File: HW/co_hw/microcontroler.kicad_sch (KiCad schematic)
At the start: 26 parts, among them J2 DS18B20, J3 DS18B20, J4 PRESSURE_SENSOR, J5 PWM, J7 Programmer, SW1 RotaryEncoder_Switch, SW2 SW_DIP_x03, SW3 SW_Push, U1 STM32F103C8Tx, U6 W25Q32JVSS, Y1 8Mhz

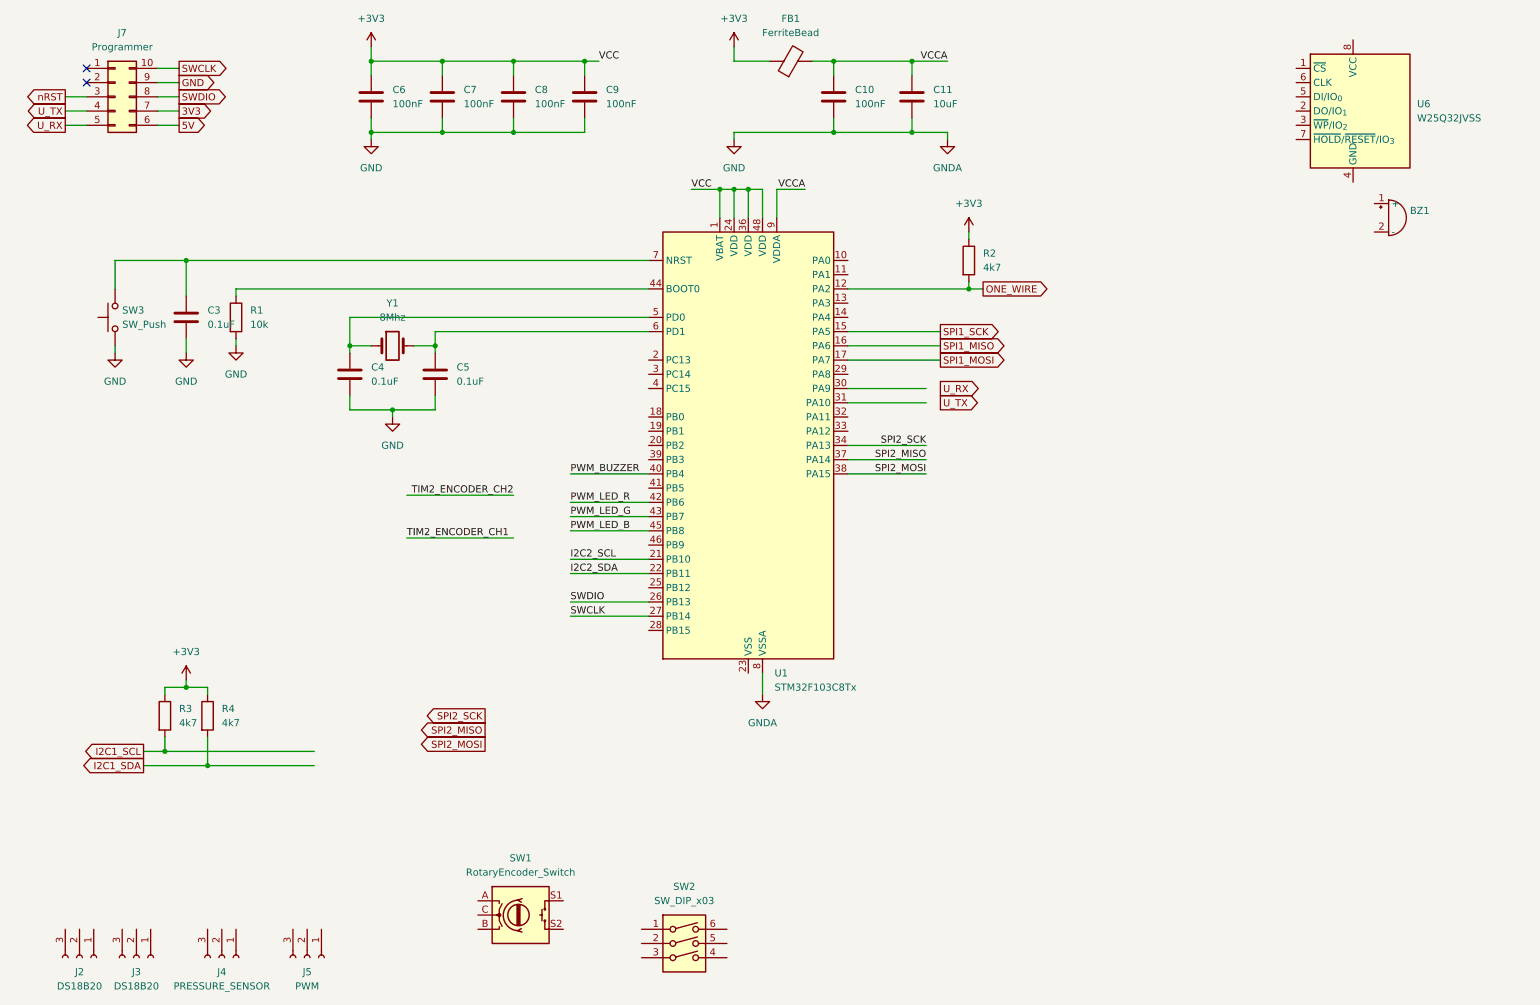
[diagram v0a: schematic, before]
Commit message: HW update.
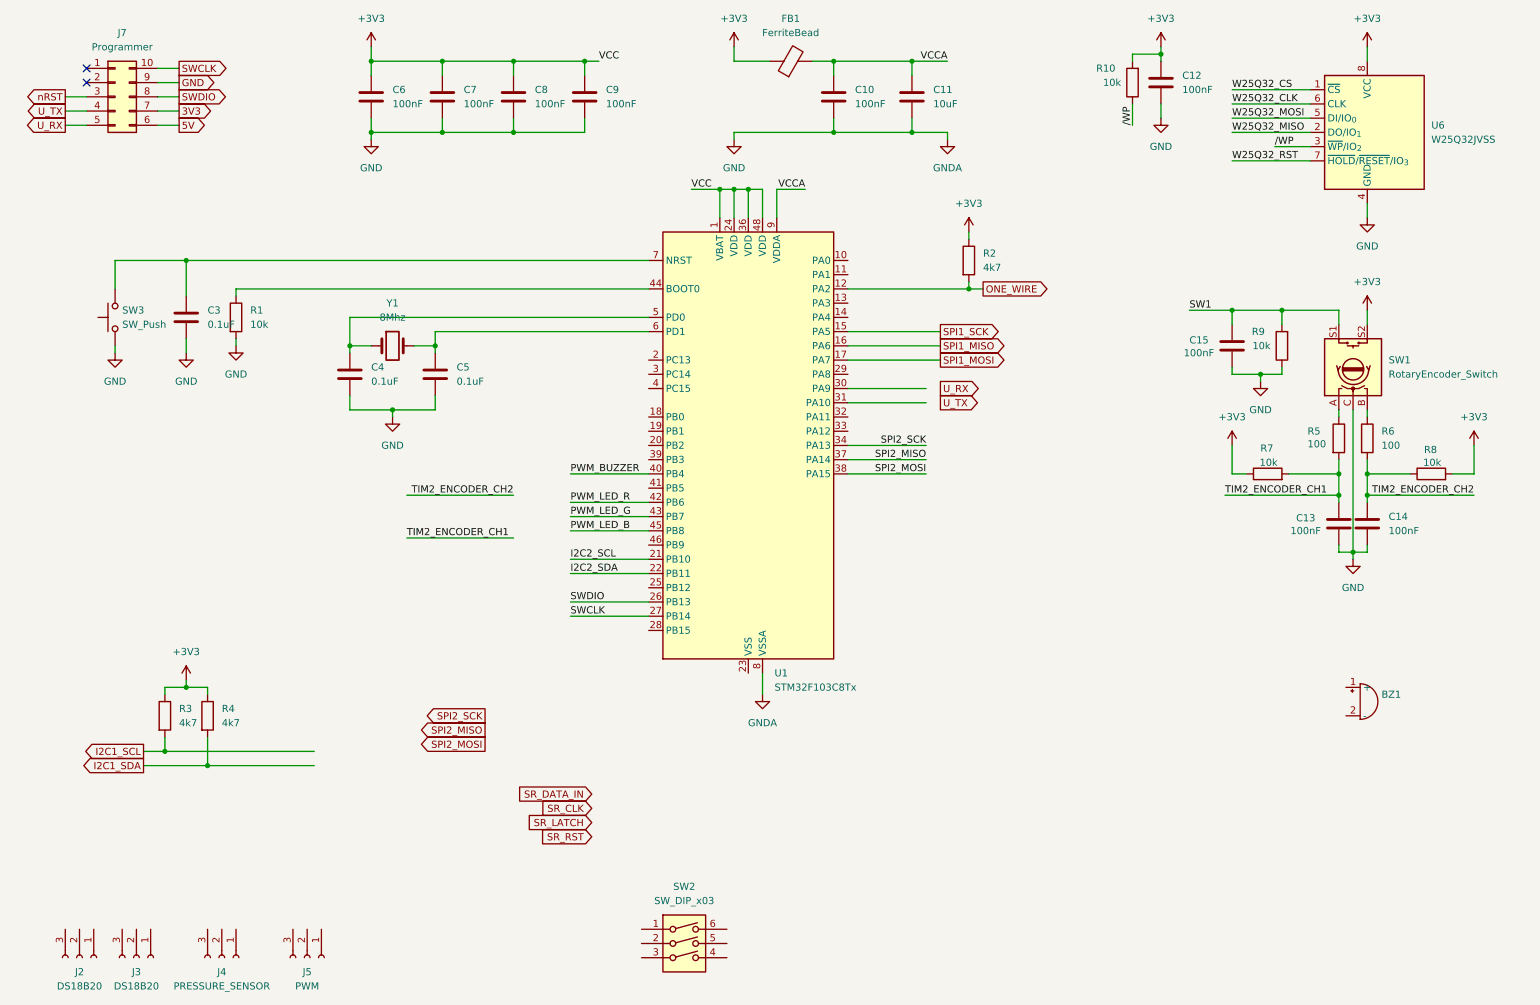
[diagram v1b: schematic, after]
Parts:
- added C12, C13, C14, C15: 100nF, symbol Device:C
- added R10, R7, R8, R9: 10k, symbol Device:R
- added R5, R6: 100, symbol Device:R
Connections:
- net +3V3: now also SW1.S2, U6.8 (VCC), C12.1, R10.2, R7.1, R8.2
- net GND: now also SW1.C, U6.4 (GND), C12.2, C13.2, C14.2, C15.2, R9.1
- net TIM2_ENCODER_CH1: now also C13.1, R5.2, R7.2
- net TIM2_ENCODER_CH2: now also C14.1, R6.2, R8.1
- net W25Q32_CS: now reaches U6.1 (~{CS})
- net W25Q32_MISO: now reaches U6.2 (DO/IO_{1})
- net /WP: now reaches U6.3 (~{WP}/IO_{2})
- net /WP: now also R10.1
- net W25Q32_MOSI: now reaches U6.5 (DI/IO_{0})
- net W25Q32_CLK: now reaches U6.6 (CLK)
- net W25Q32_RST: now reaches U6.7 (~{HOLD}/~{RESET}/IO_{3})
- net at SW1.A: now also R5.1
- net at SW1.B: now also R6.1
- net SW1: now reaches SW1.S1
- net SW1: now also C15.1, R9.2
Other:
- moved on the sheet: BZ1, SW1, U6

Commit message: HW update.
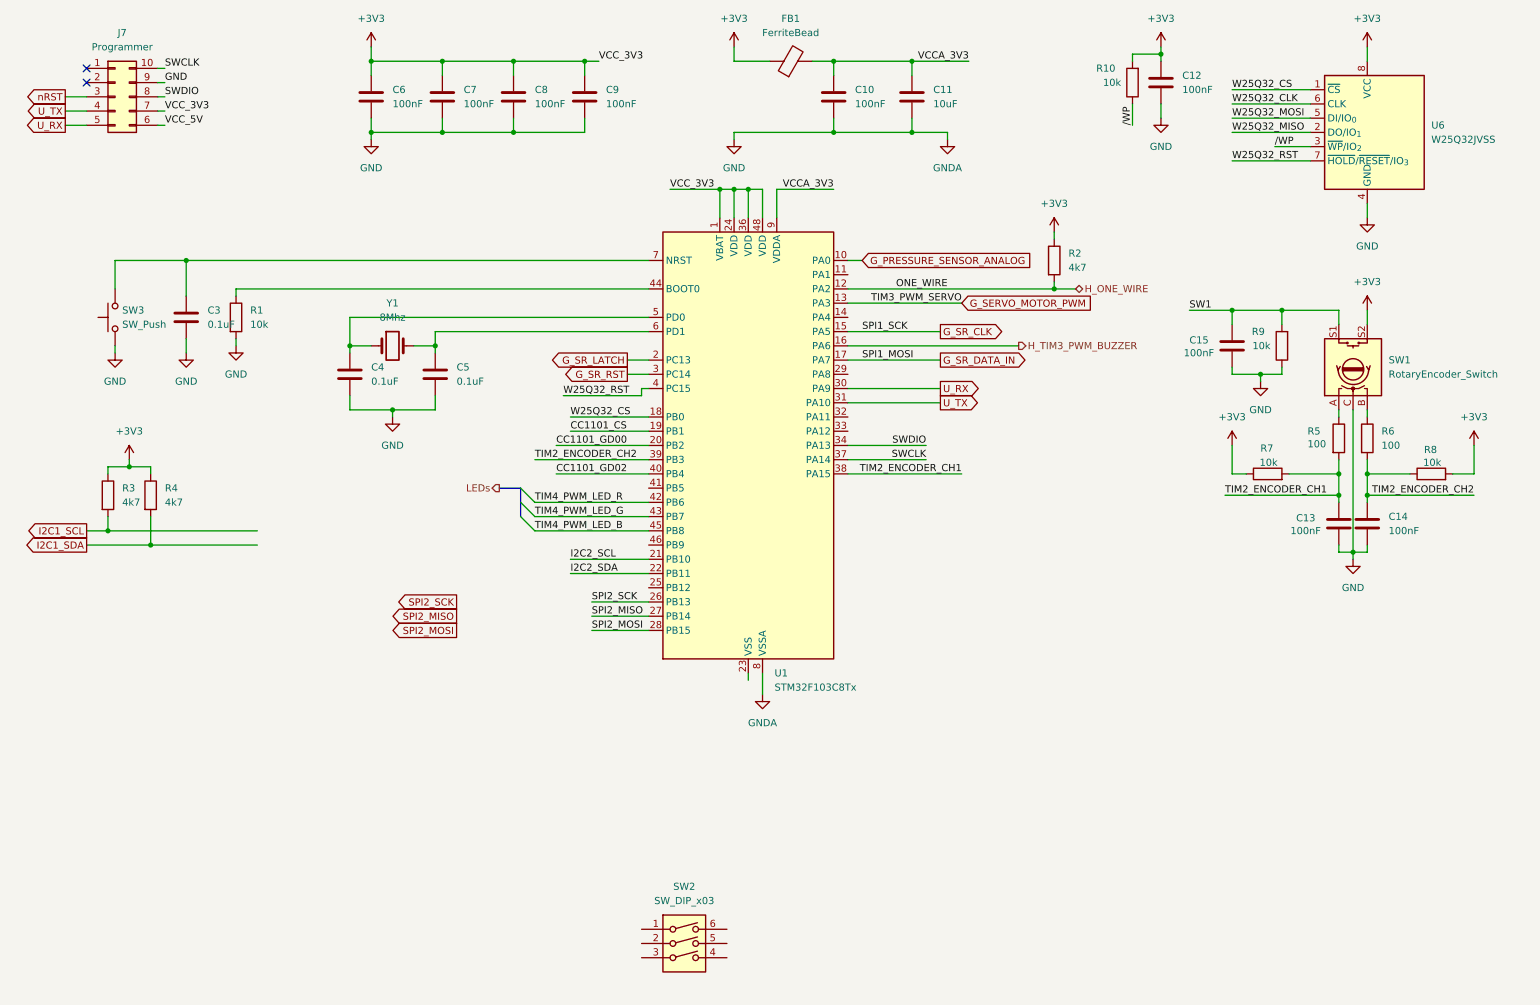
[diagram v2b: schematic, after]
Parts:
- removed BZ1: ~, Own_Library:SFM-27-W, symbol Own_Library:SFM-27
- removed J2: DS18B20, Connector_Molex:Molex_Mini-Fit_Sr_42820-32XX_1x03_P10.00mm_Horizontal_ThermalVias, symbol Connector:Conn_01x03_Socket
- removed J3: DS18B20, symbol Connector:Conn_01x03_Socket
- removed J4: PRESSURE_SENSOR, symbol Connector:Conn_01x03_Socket
- removed J5: PWM, symbol Connector:Conn_01x03_Socket
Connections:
- net 3V3 is gone; now on net +3V3: J7.7 (Pin_7)
- net SPI2_MISO: now also U1.27 (PB14); no longer U1.37 (PA14)
- net SPI2_MOSI: now also U1.28 (PB15); no longer U1.38 (PA15)
- net SPI2_SCK: now also U1.26 (PB13); no longer U1.34 (PA13)
- net SWCLK: now also U1.37 (PA14); no longer U1.27 (PB14)
- net SWDIO: now also U1.34 (PA13); no longer U1.26 (PB13)
- net TIM2_ENCODER_CH1: now also U1.38 (PA15)
- net TIM2_ENCODER_CH2: now also U1.39 (PB3)
- net U_RX: now also U1.30 (PA9)
- net U_TX: now also U1.31 (PA10)
- net W25Q32_CS: now also U1.18 (PB0)
- net W25Q32_RST: now also U1.4 (PC15)
- net G_PRESSURE_SENSOR_ANALOG: now reaches U1.10 (PA0)
- net G_SERVO_MOTOR_PWM: now reaches U1.13 (PA3)
- net CC1101_CS: now reaches U1.19 (PB1)
- net G_SR_LATCH: now reaches U1.2 (PC13)
- net CC1101_GD00: now reaches U1.20 (PB2)
- net G_SR_RST: now reaches U1.3 (PC14)
- net 5V renamed VCC_5V
- net ONE_WIRE renamed H_ONE_WIRE
- net PWM_BUZZER renamed CC1101_GD02
- net PWM_LED_B renamed TIM4_PWM_LED_B
- net PWM_LED_G renamed TIM4_PWM_LED_G
- net PWM_LED_R renamed TIM4_PWM_LED_R
- net SPI1_MISO renamed H_TIM3_PWM_BUZZER
- net SPI1_MOSI renamed G_SR_DATA_IN
- net SPI1_SCK renamed G_SR_CLK
- net VCCA renamed VCCA_3V3
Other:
- moved on the sheet: R2, R3, R4
